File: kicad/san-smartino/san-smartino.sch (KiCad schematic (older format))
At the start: 49 parts, among them J1 GND CTS VBUS RX TX DTR, J2 SDA SCL -3V3 GND, J3 Conn_01x07_Male, SW1 Reset, SW2 Flash, U1 BQ27441DRZR-G1A, U2 ESP-12E, U3 LTC3440

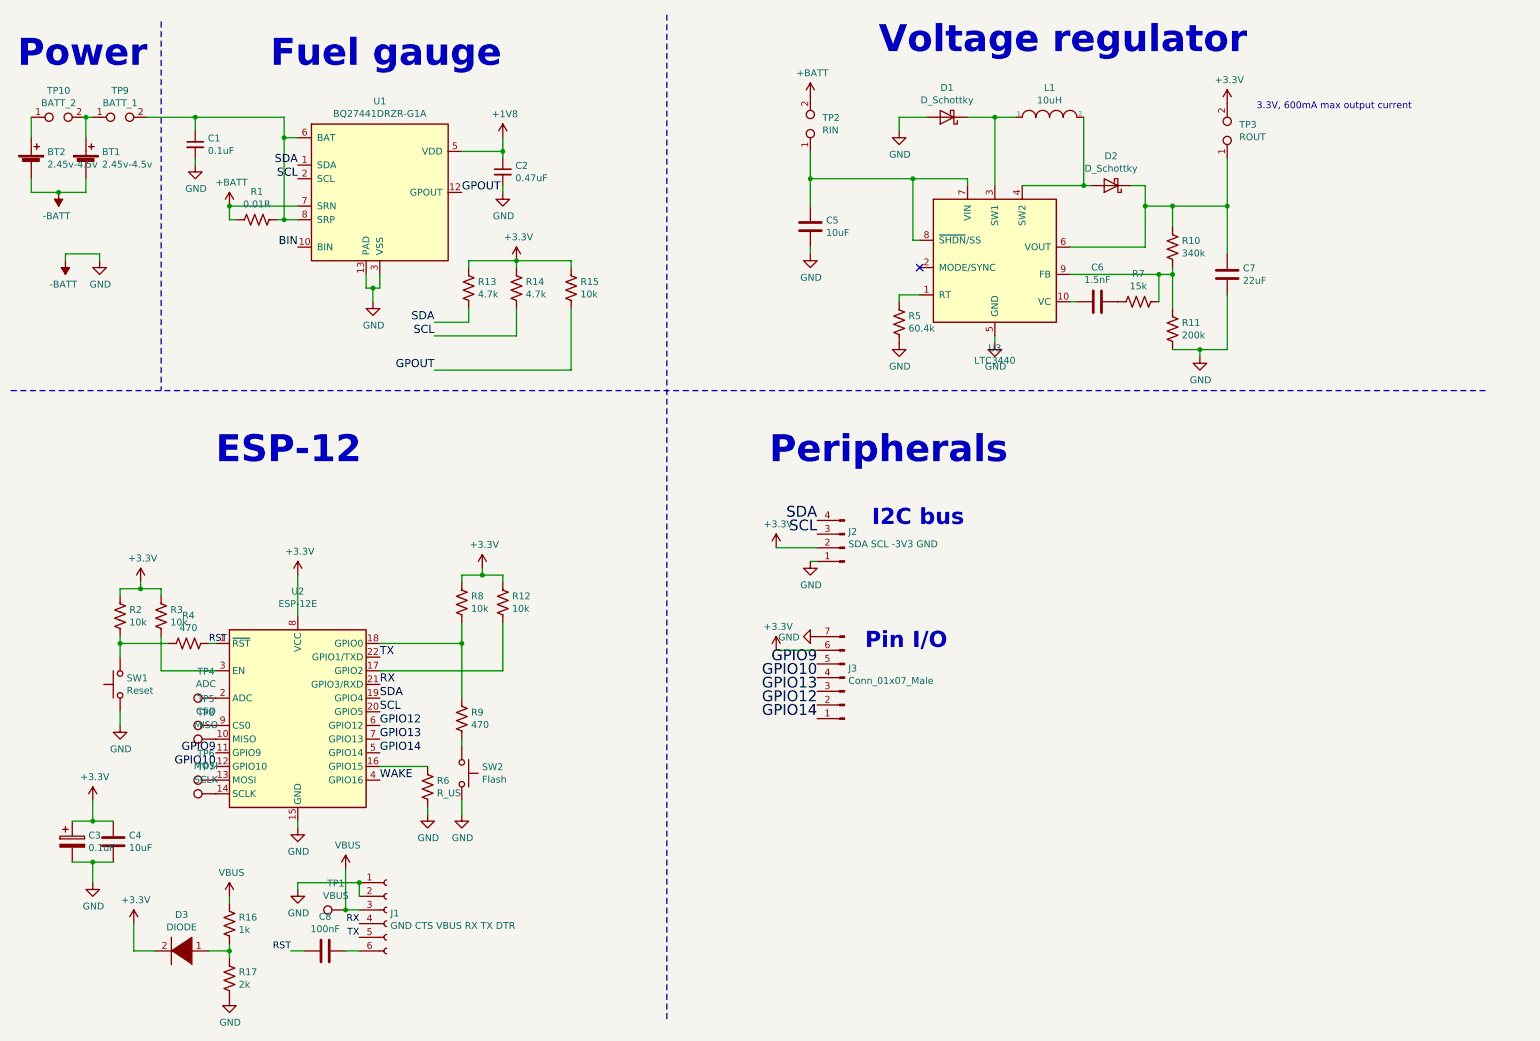
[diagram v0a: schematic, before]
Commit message: updated board
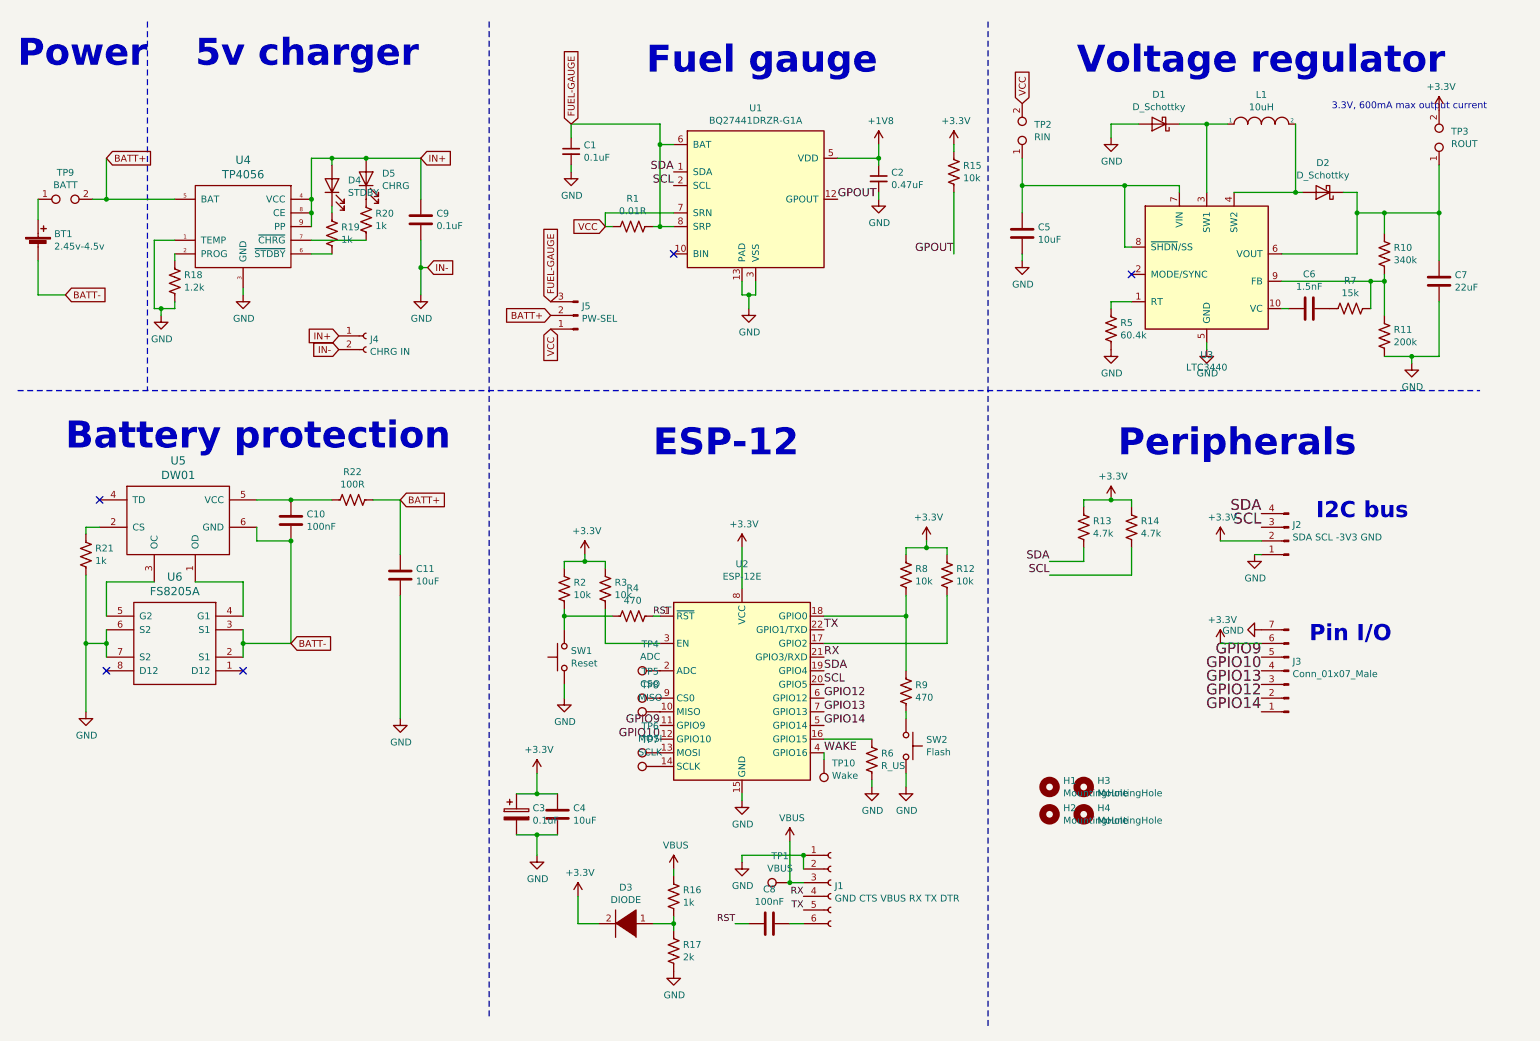
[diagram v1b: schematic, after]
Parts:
- removed BT2: 2.45v-4.5v, san-smartino:18650-battery-metal-clips, symbol Device:Battery_Cell
- removed TP10: BATT_2, TestPoint:TestPoint_2Pads_Pitch2.54mm_Drill0.8mm, symbol Connector:TestPoint_2Pole
- added C10: 100nF, Capacitor_SMD:C_0805_2012Metric_Pad1.15x1.40mm_HandSolder, symbol Device:C
- added C11: 10uF, Capacitor_SMD:C_0805_2012Metric_Pad1.15x1.40mm_HandSolder, symbol Device:C
- added C9: 0.1uF, Capacitor_SMD:C_0805_2012Metric_Pad1.15x1.40mm_HandSolder, symbol Device:C
- added D4: STDBY, LED_SMD:LED_0603_1608Metric_Pad1.05x0.95mm_HandSolder, symbol Device:LED
- added D5: CHRG, LED_SMD:LED_0603_1608Metric_Pad1.05x0.95mm_HandSolder, symbol Device:LED
- added H1, H2, H3, H4: MountingHole, MountingHole:MountingHole_3.2mm_M3_Pad_Via, symbol Mechanical:MountingHole
- added J4: CHRG IN, Connector_PinHeader_2.54mm:PinHeader_1x02_P2.54mm_Vertical, symbol Connector:Conn_01x02_Female
- added J5: PW-SEL, Connector_PinHeader_2.54mm:PinHeader_1x03_P2.54mm_Vertical, symbol Connector:Conn_01x03_Male
- added R18: 1.2k, Resistor_SMD:R_0805_2012Metric_Pad1.15x1.40mm_HandSolder, symbol Device:R_US
- added R19, R20, R21: 1k, Resistor_SMD:R_0805_2012Metric_Pad1.15x1.40mm_HandSolder, symbol Device:R_US
- added R22: 100R, Resistor_SMD:R_0805_2012Metric_Pad1.15x1.40mm_HandSolder, symbol Device:R_US
- added TP10: Wake, TestPoint:TestPoint_Pad_D1.5mm, symbol Connector:TestPoint
- added U4: TP4056, Package_SO:SOP-8-1EP_4.57x4.57mm_P1.27mm_EP4.57x4.45mm, symbol tp4056:TP4056
- added U5: DW01, Package_TO_SOT_SMD:SOT-23-6_Handsoldering, symbol dw01:DW01
- added U6: FS8205A, Package_SO:TSSOP-8_4.4x3mm_P0.65mm, symbol fs8205a:FS8205A
- SW1: footprint Button_Switch_SMD:SW_SPST_CK_RS282G05A3 -> Button_Switch_SMD:SW_SPST_EVQP0
- TP9: value BATT_1 -> BATT
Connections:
- net WAKE: now also TP10.1
- net FUEL-GAUGE: now reaches C1.1, R1.1, U1.6 (BAT), U1.8 (SRP)
- net FUEL-GAUGE: now also J5.3 (Pin_3); no longer TP9.2
- net +BATT renamed VCC
- net VCC: now also J5.1 (Pin_1)
- net -BATT renamed GND
- net GND: now also C11.2, C9.2, J4.2 (Pin_2), R18.2, R21.2, U4.1 (TEMP), U4.3 (GND), U6.6 (S2), U6.7 (S2); no longer BT1.2 (-)
- net BIN: no longer names the net of U1.10 (BIN)
- new net: R18.1, U4.2 (PROG)
- new net: R19.2, U4.6 (~STDBY)
- new net: R20.2, U4.7 (~CHRG)
- new net: D4.1 (K), R19.1
- new net: D5.1 (K), R20.1
- new net: U5.1 (OD), U6.4 (G1)
- new net: R21.1, U5.2 (CS)
- new net: U5.3 (OC), U6.5 (G2)
- new net: C10.1, R22.2, U5.5 (VCC)
- new net BATT+: C11.1, J5.2 (Pin_2), R22.1, TP9.2, U4.5 (BAT)
- new net BATT-: BT1.2 (-), C10.2, U5.6 (GND), U6.2 (S1), U6.3 (S1)
- new net IN+: C9.1, D4.2 (A), D5.2 (A), J4.1 (Pin_1), U4.4 (VCC), U4.8 (CE), U4.9 (PP)
- no-connect marks 1 -> 5
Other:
- note added: "5v charger"
- note added: "Battery protection"
- moved on the sheet: BT1, C1, C2, C3, C4, C5, C6, C7, C8, D1, D2, D3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
